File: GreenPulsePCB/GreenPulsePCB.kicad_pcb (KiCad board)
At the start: 2 copper layers, 26 x 25 mm, 23 parts, among them J1 Conn_01x05, J2 Conn_01x02, Q1 NPN, Q2 NPN, Q3 NPN, Q4 NPN, U1 BME280

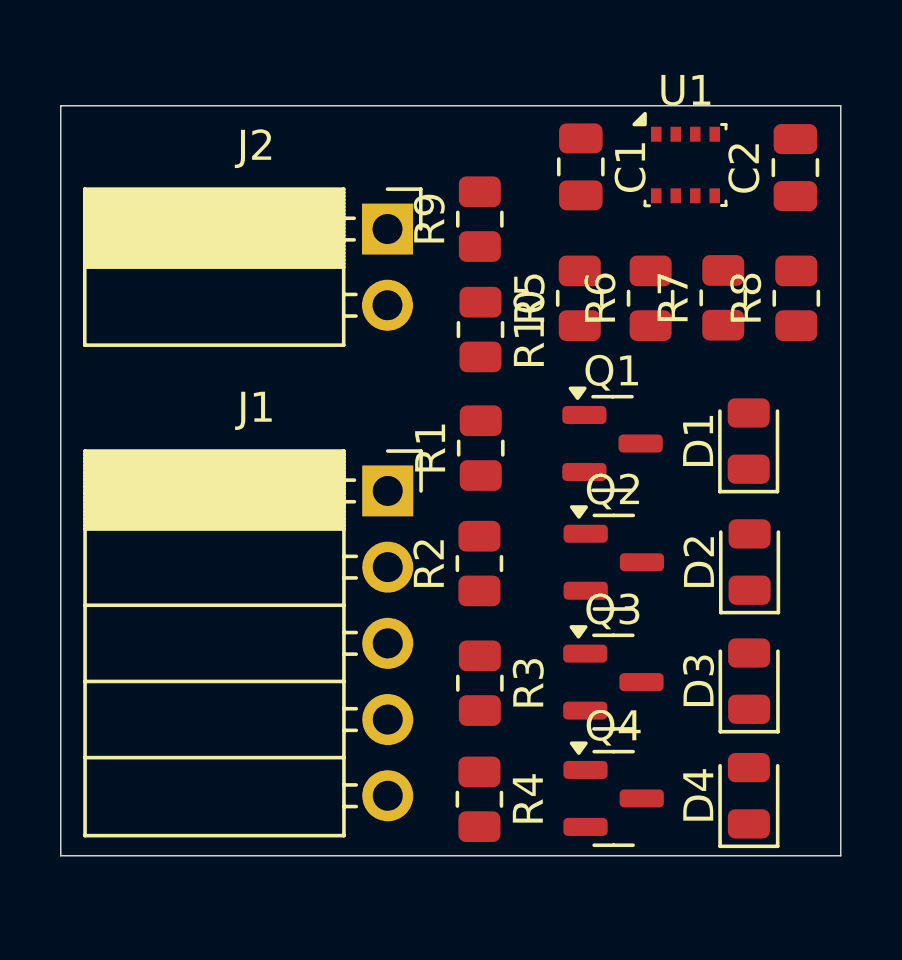
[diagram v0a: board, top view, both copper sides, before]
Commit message: Routing abgeschlossen
Kann trotzdem noch Fehler beinhalten. Nochmal gründlich überprüfen!
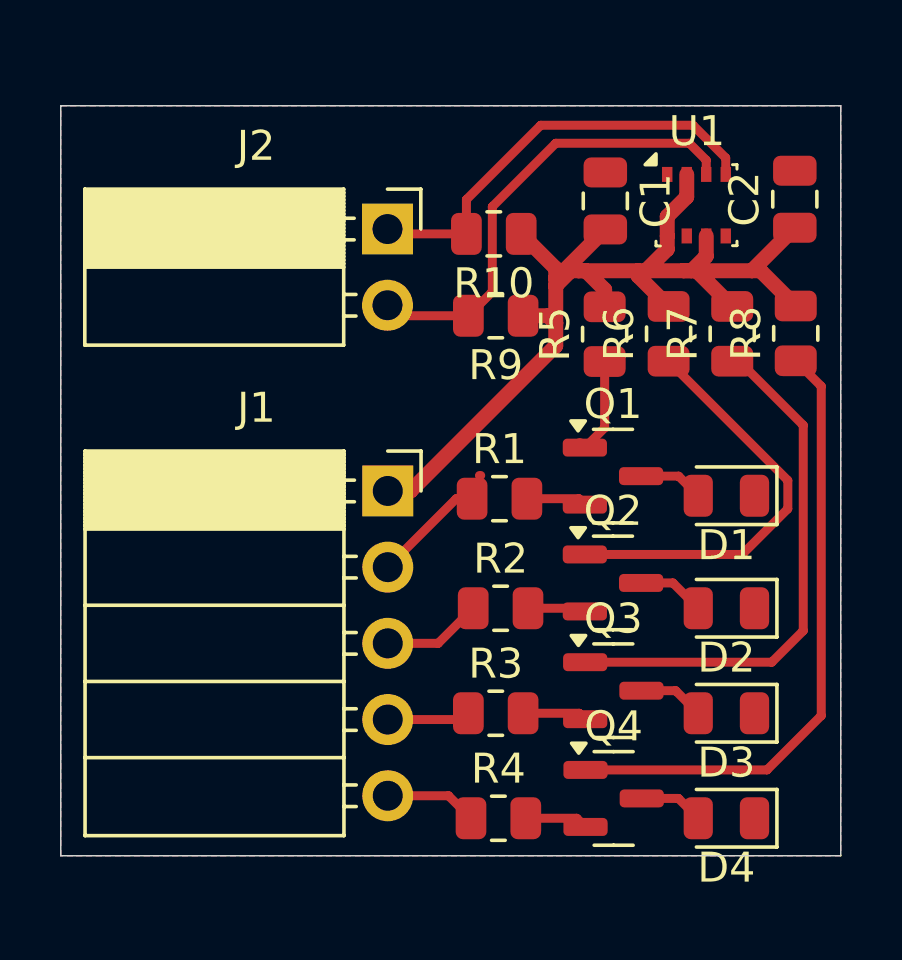
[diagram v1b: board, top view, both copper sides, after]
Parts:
- moved R9 3.26 mm to (91.5, 33.5), turned to 180 degrees
- moved R10 3.22 mm to (91.4, 30.8), turned to 180 degrees
- moved D1 1.97 mm to (99.2, 39.5), turned to 180 degrees
- moved R1 1.80 mm to (91.6, 39.6), turned to 0 degrees
- moved D2 1.72 mm to (99.2, 43.2), turned to 180 degrees
- moved R2 1.65 mm to (91.7, 43.2), turned to 0 degrees
- moved R5 1.46 mm to (95.1, 34.1)
- moved C1 1.40 mm to (95.2, 29.7)
- moved U1 1.39 mm to (98.2, 29.8)
- moved R6 1.33 mm to (97.3, 34.1)
- moved D3 1.31 mm to (99.2, 46.8), turned to 180 degrees
- moved R7 1.24 mm to (99.4, 34.1)
- moved R8 1.17 mm to (101.5, 34.1)
- moved R3 1.13 mm to (91.5, 46.8), turned to 0 degrees
- moved Q1 1.09 mm to (95.4, 38.8)
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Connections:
- J2 pad 1: OUT2 -> OUT1
- J2 pad 2: OUT1 -> OUT2
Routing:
- net 3,3V: track 0.00 -> 36.6 mm
- net Net-(Q4-C): track 0.00 -> 20.8 mm
- net Net-(Q3-C): track 0.00 -> 17.8 mm
- net OUT2: track 0.00 -> 15.5 mm
- net OUT1: track 0.00 -> 14.5 mm
- net Net-(Q2-C): track 0.00 -> 14.0 mm
- net IN1: track 0.00 -> 3.80 mm
- net Net-(Q1-C): track 0.00 -> 3.38 mm
- net IN2: track 0.00 -> 3.33 mm
- net IN4: track 0.00 -> 3.09 mm
- net IN3: track 0.00 -> 2.77 mm
- net Net-(D2-A): track 0.00 -> 2.25 mm
- net Net-(D3-A): track 0.00 -> 2.20 mm
- net Net-(D1-A): track 0.00 -> 2.18 mm
- net Net-(D4-A): track 0.00 -> 2.16 mm
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- added copper zone on B.Cu, net GND
- added copper zone on F.Cu, net GND
